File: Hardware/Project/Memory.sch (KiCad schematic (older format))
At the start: 4 parts, among them U17 28C256, U5 74LS138, U6 28C256, U7 28C256

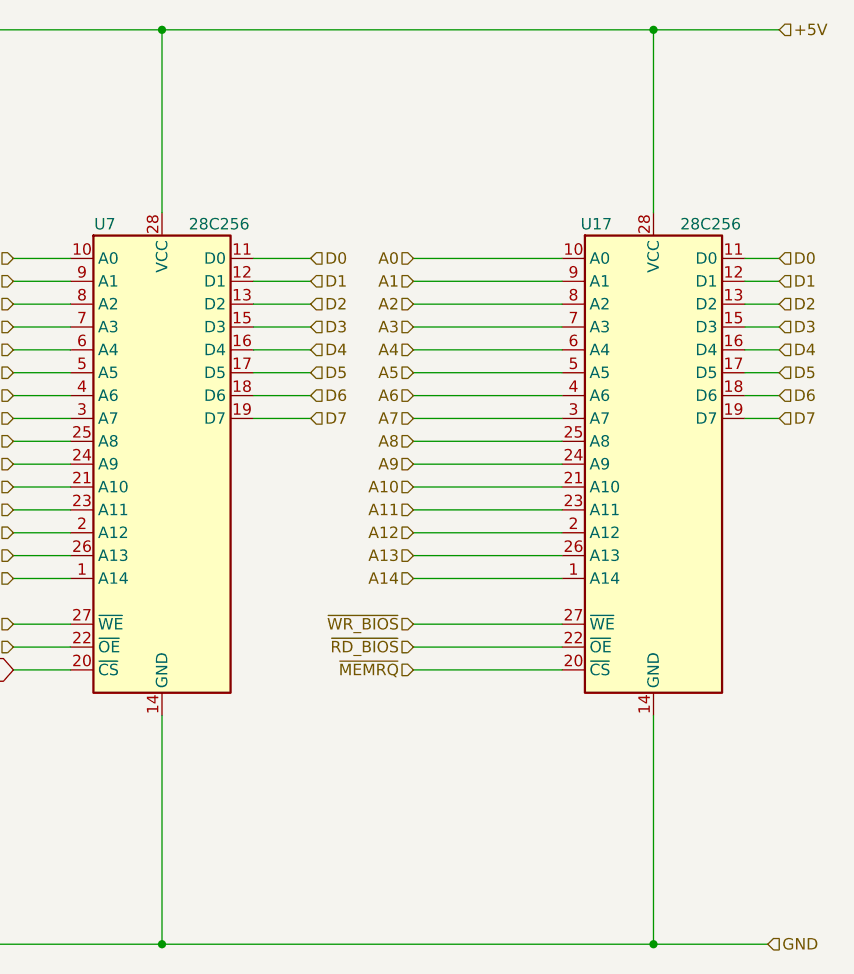
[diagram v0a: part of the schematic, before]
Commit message: 1
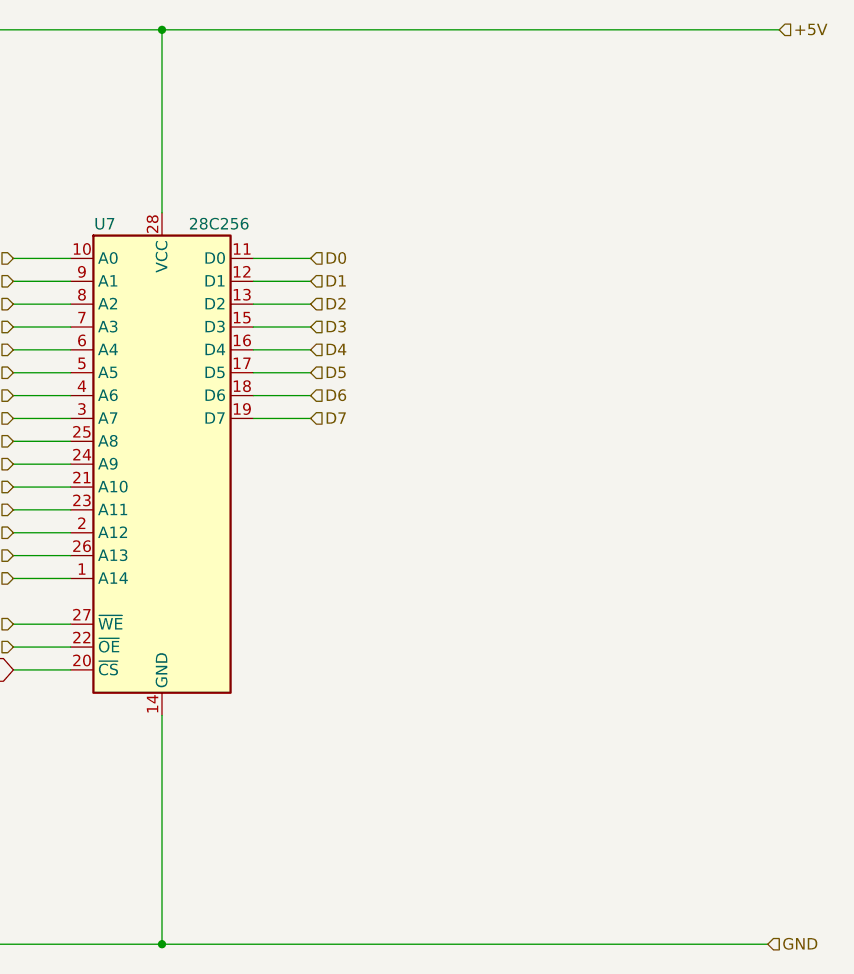
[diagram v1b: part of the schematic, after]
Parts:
- removed U17: 28C256, Package_DIP:DIP-28_W15.24mm_Socket, symbol Memory_EEPROM:28C256
- U5: footprint Package_DIP:DIP-18_W7.62mm_Socket -> Package_DIP:DIP-16_W7.62mm_Socket
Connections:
- net labels removed: ~RD_BIOS, ~WR_BIOS
- wire segments 117 -> 87
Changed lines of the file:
@@
 $Descr A4 11693 8268
 encoding utf-8
-Sheet 4 6
+Sheet 3 5
 Title ""
 Date ""
@@
 F 0 "U5" H 2500 3300 50  0000 C CNN
 F 1 "74LS138" H 3000 3300 50  0000 C CNN
-F 2 "Package_DIP:DIP-18_W7.62mm_Socket" H 2750 2850 50  0001 C CNN
+F 2 "Package_DIP:DIP-16_W7.62mm_Socket" H 2750 2850 50  0001 C CNN
 F 3 "http://www.ti.com/lit/gpn/sn74LS138" H 2750 2850 50  0001 C CNN
 	1    2750 2850
@@
 Connection ~ 6650 950
 Connection ~ 6650 4950
-Wire Wire Line
-	6650 4950 8800 4950
-Wire Wire Line
-	6650 950  8800 950
 Text GLabel 4200 3750 0    50   Input ~ 0
 ~MEM0_CS
@@
 Wire Wire Line
 	2750 3600 2750 4950
-$Comp
-L Memory_EEPROM:28C256 U?
-U 1 1 5DBEF611
-P 8800 2850
-AR Path="/5C68B4BB/5DBEF611" Ref="U?"  Part="1"
-AR Path="/5DED3C2A/5DBEF611" Ref="U?"  Part="1"
-AR Path="/5E17A1DA/5DBEF611" Ref="U17"  Part="1"
-F 0 "U17" H 8550 3900 50  0000 C CNN
-F 1 "28C256" H 9050 3900 50  0000 C CNN
-F 2 "Package_DIP:DIP-28_W15.24mm_Socket" H 8800 2850 50  0001 C CNN
-F 3 "http://ww1.microchip.com/downloads/en/DeviceDoc/doc0006.pdf" H 8800 2850 50  0001 C CNN
-	1    8800 2850
-	1    0    0    -1
-$EndComp
-Wire Wire Line
-	8400 3350 7750 3350
-Wire Wire Line
-	8400 3250 7750 3250
-Wire Wire Line
-	8400 3150 7750 3150
-Wire Wire Line
-	8400 3050 7750 3050
-Wire Wire Line
-	8400 2950 7750 2950
-Wire Wire Line
-	8400 2850 7750 2850
-Wire Wire Line
-	8400 2750 7750 2750
-Text HLabel 7750 3350 0    50   Input ~ 0
-A14
-Text HLabel 7750 3250 0    50   Input ~ 0
-A13
-Text HLabel 7750 3150 0    50   Input ~ 0
-A12
-Text HLabel 7750 3050 0    50   Input ~ 0
-A11
-Text HLabel 7750 2950 0    50   Input ~ 0
-A10
-Text HLabel 7750 2850 0    50   Input ~ 0
-A9
-Text HLabel 7750 2750 0    50   Input ~ 0
-A8
-Wire Wire Line
-	8400 2650 7750 2650
-Wire Wire Line
-	7750 2550 8400 2550
-Wire Wire Line
-	8400 2450 7750 2450
-Wire Wire Line
-	7750 2350 8400 2350
-Wire Wire Line
-	8400 2250 7750 2250
-Wire Wire Line
-	7750 2150 8400 2150
-Wire Wire Line
-	8400 2050 7750 2050
-Text HLabel 7750 2650 0    50   Input ~ 0
-A7
-Text HLabel 7750 2550 0    50   Input ~ 0
-A6
-Text HLabel 7750 2450 0    50   Input ~ 0
-A5
-Text HLabel 7750 2350 0    50   Input ~ 0
-A4
-Text HLabel 7750 2250 0    50   Input ~ 0
-A3
-Text HLabel 7750 2150 0    50   Input ~ 0
-A2
-Text HLabel 7750 2050 0    50   Input ~ 0
-A1
-Text HLabel 7750 1950 0    50   Input ~ 0
-A0
-Wire Wire Line
-	8400 1950 7750 1950
-Text HLabel 9350 2650 2    50   Input ~ 0
-D7
-Text HLabel 9350 2550 2    50   Input ~ 0
-D6
-Text HLabel 9350 2450 2    50   Input ~ 0
-D5
-Text HLabel 9350 2350 2    50   Input ~ 0
-D4
-Text HLabel 9350 2250 2    50   Input ~ 0
-D3
-Text HLabel 9350 2150 2    50   Input ~ 0
-D2
-Text HLabel 9350 2050 2    50   Input ~ 0
-D1
-Text HLabel 9350 1950 2    50   Input ~ 0
-D0
-Wire Wire Line
-	9350 1950 9200 1950
-Wire Wire Line
-	9350 2050 9200 2050
-Wire Wire Line
-	9350 2150 9200 2150
-Wire Wire Line
-	9350 2250 9200 2250
-Wire Wire Line
-	9350 2350 9200 2350
-Wire Wire Line
-	9350 2450 9200 2450
-Wire Wire Line
-	9350 2550 9200 2550
-Wire Wire Line
-	9350 2650 9200 2650
-Wire Wire Line
-	7750 3550 8400 3550
-Wire Wire Line
-	8400 3650 7750 3650
-Wire Wire Line
-	8800 950  8800 1750
-Text HLabel 7750 3750 0    50   Input ~ 0
-~MEMRQ
-Wire Wire Line
-	8800 3950 8800 4950
-Wire Wire Line
-	7750 3750 8400 3750
-Text HLabel 7750 3650 0    50   Input ~ 0
-~RD_BIOS
-Text HLabel 7750 3550 0    50   Input ~ 0
-~WR_BIOS
-Connection ~ 8800 950
-Connection ~ 8800 4950
-Wire Wire Line
-	8800 4950 9300 4950
-Wire Wire Line
-	8800 950  9350 950
+Wire Wire Line
+	6650 950  9350 950
+Wire Wire Line
+	6650 4950 9300 4950
 $EndSCHEMATC
